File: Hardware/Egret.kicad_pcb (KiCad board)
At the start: 2 copper layers, 92 x 37.2 mm, 45 parts, among them J1 Conn_01x20_Male, J2 Conn_01x20_Male, J3 USB_B_Micro, Q1 S8050, Q2 S8050, SW1 SW_Push, SW2 SW_Push, U1 AMS1117-3.3, U2 ESP32-PICO-D4, U3 CP2102N-A01-GQFN28

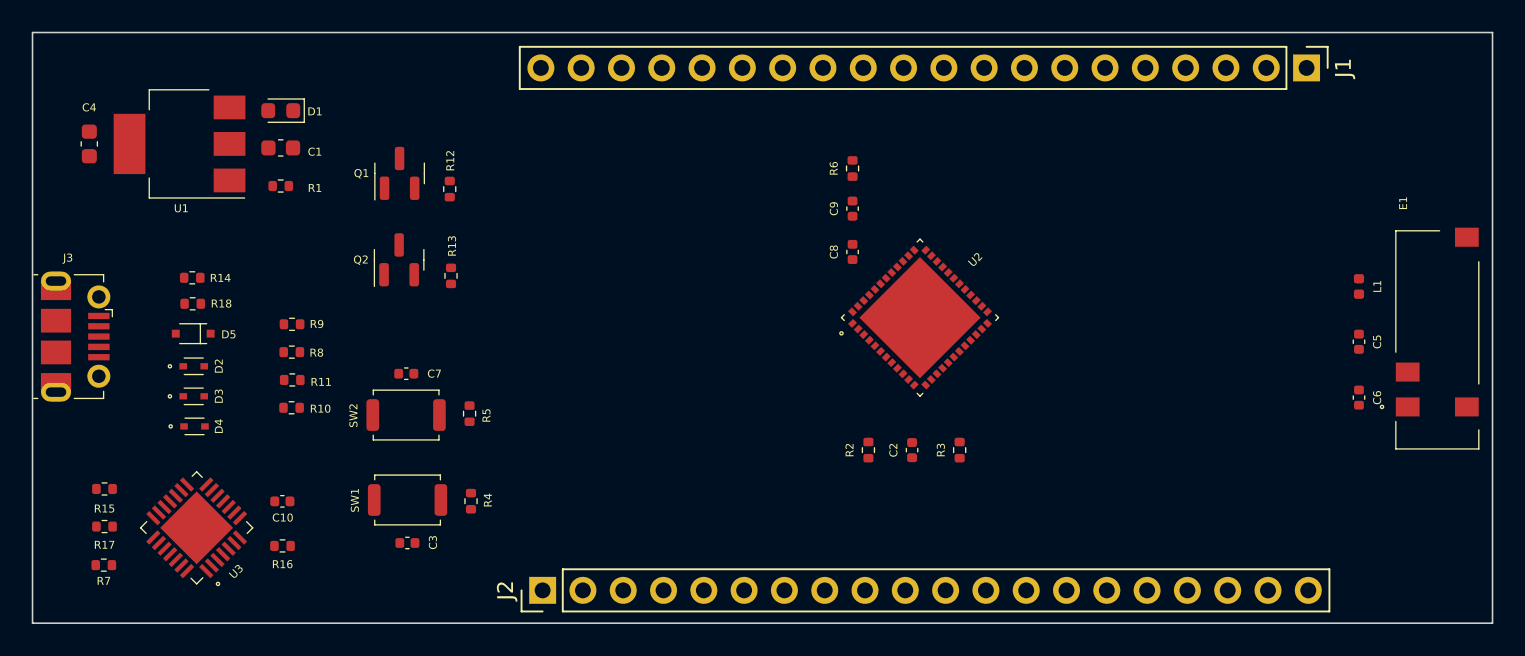
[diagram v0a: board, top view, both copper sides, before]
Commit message: update PCB
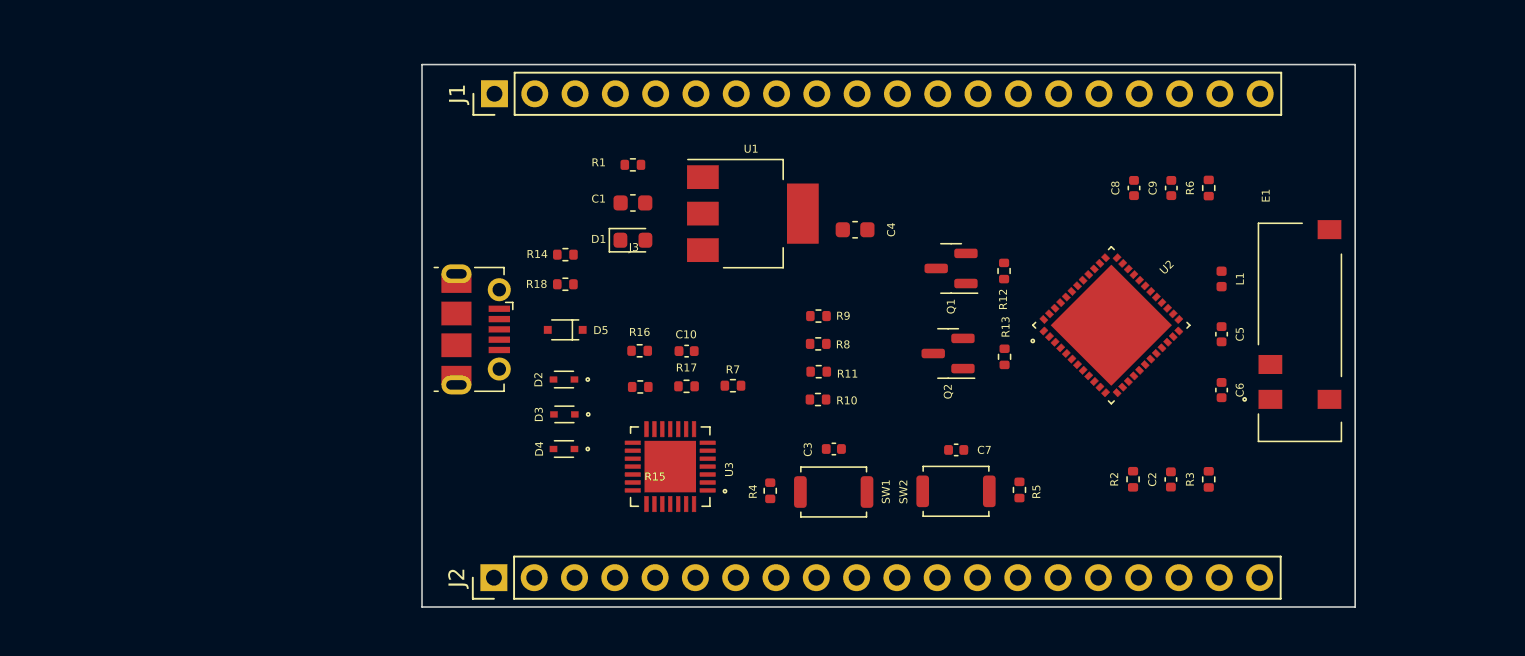
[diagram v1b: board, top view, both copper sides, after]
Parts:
- moved J1 51.2 mm to (152.7, 52.5), turned to 90 degrees
- moved C4 48.6 mm to (175.4, 61.1), turned to 180 degrees
- moved R7 41.2 mm to (167.7, 70.9), turned to 0 degrees
- moved R17 37.7 mm to (164.8, 71.0), turned to 0 degrees
- moved U1 36.4 mm to (169.0, 60.1), turned to 0 degrees
- moved R12 35.3 mm to (184.8, 63.7), turned to -90 degrees
- moved Q1 35.3 mm to (181.4, 63.5), turned to 180 degrees
- moved R13 35.3 mm to (184.8, 69.1)
- moved Q2 35.1 mm to (181.3, 68.9), turned to 180 degrees
- moved C7 35.0 mm to (181.8, 75.0)
- moved R5 35.0 mm to (185.8, 77.5)
- moved SW2 35.0 mm to (181.8, 77.6)
- moved R15 34.4 mm to (161.9, 71.0)
- moved R10 33.2 mm to (173.1, 71.8)
- moved R11 33.2 mm to (173.1, 70.0)
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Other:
- board size 92 x 37.2 mm -> 58.8 x 34.2 mm
